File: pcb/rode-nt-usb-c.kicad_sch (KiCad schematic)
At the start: 6 parts, among them J1 USB_C_Receptacle_USB2.0_16P, J2 Conn_01x05_Pin

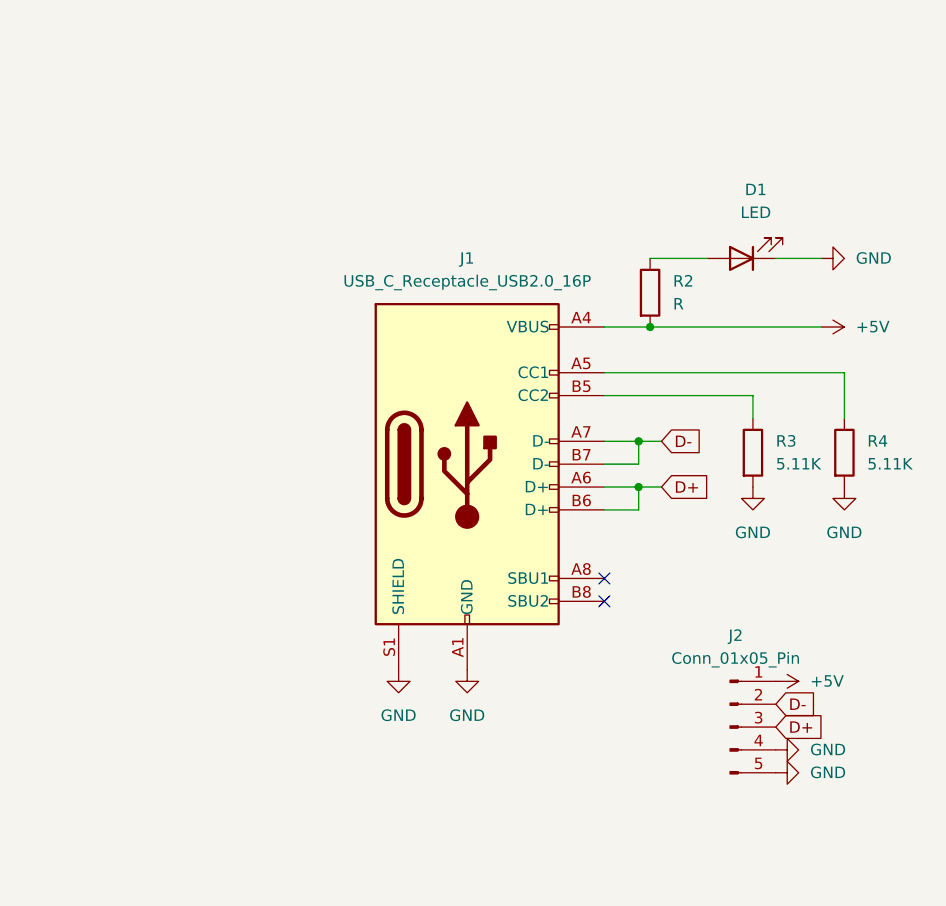
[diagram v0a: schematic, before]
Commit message: Change design, multiple adjustments
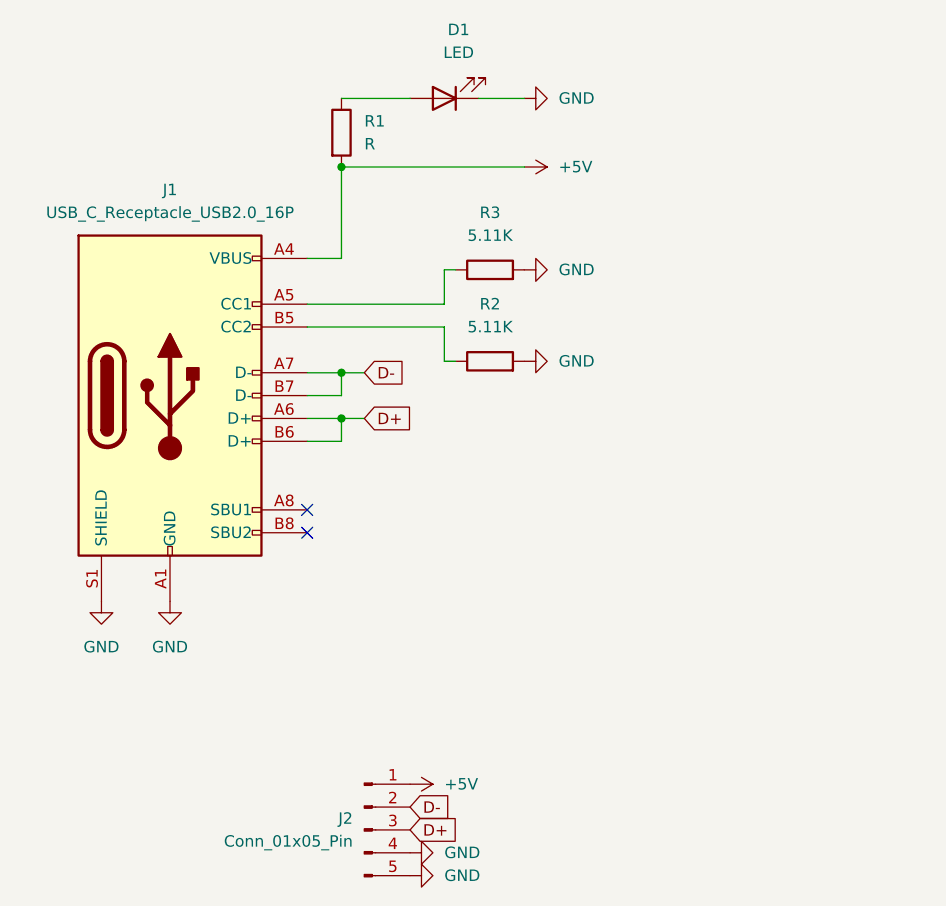
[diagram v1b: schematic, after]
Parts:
- renumbered R2 to R1, R3 to R2, R4 to R3
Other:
- title: (none) -> RODE NT-USB-C
- moved on the sheet: D1, J1, J2, R1, R2, R3
